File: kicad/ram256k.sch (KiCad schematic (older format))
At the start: 11 parts

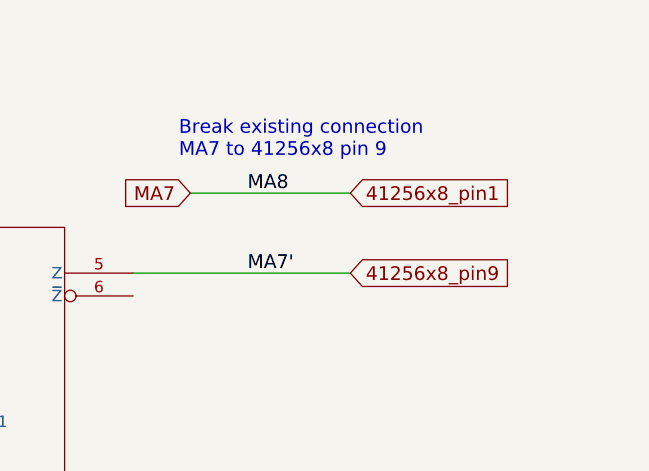
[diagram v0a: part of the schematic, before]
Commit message: Minor schematic update
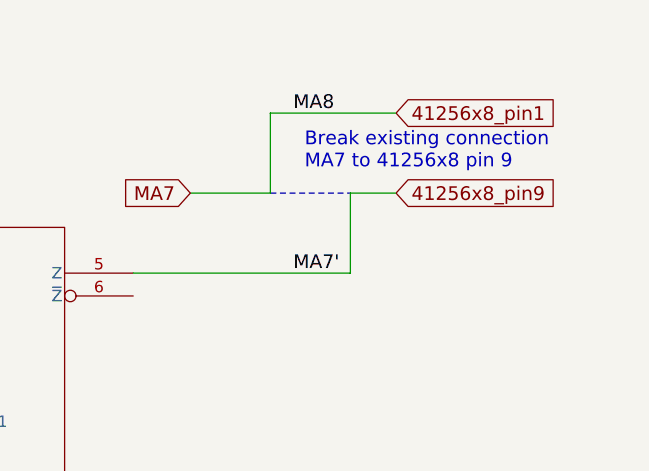
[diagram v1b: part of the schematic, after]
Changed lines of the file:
@@
 Wire Wire Line
 	7000 3350 9650 3350
-Text GLabel 9650 1600 2    60   Input ~ 0
+Text GLabel 9850 1250 2    60   Input ~ 0
 41256x8_pin1
 Wire Wire Line
@@
 Text Label 6400 1350 0    60   ~ 0
 RA7
-Text Label 9200 1950 0    60   ~ 0
+Text Label 9400 1950 0    60   ~ 0
 MA7'
-Text GLabel 9650 1950 2    60   Input ~ 0
+Text GLabel 9850 1600 2    60   Input ~ 0
 41256x8_pin9
 Text GLabel 8950 1600 0    60   Input ~ 0
 MA7
-Wire Wire Line
-	8950 1600 9650 1600
-Text Label 9200 1600 0    60   ~ 0
+Text Label 9400 1250 0    60   ~ 0
 MA8
-Text Notes 8900 1450 0    60   ~ 0
+Text Notes 9450 1500 0    60   ~ 0
 Break existing connection\nMA7 to 41256x8 pin 9
+Wire Wire Line
+	9650 1950 9650 1600
+Wire Wire Line
+	9650 1600 9850 1600
+Wire Wire Line
+	8950 1600 9300 1600
+Wire Wire Line
+	9300 1600 9300 1250
+Wire Wire Line
+	9300 1250 9850 1250
+Wire Notes Line
+	9300 1600 9650 1600
 $EndSCHEMATC
